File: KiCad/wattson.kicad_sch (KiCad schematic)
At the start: 24 parts, among them SW1 Keypad 1, SW10 Plug, SW11 On/Off, SW2 Keypad 2, SW3 Keypad 3, SW4 Keypad 4, SW5 Keypad 5, SW6 Keypad 0, SW7 Keypad 6, SW8 Keypad 7, SW9 Trigger, U1 CR2013-MI2120, U2 MCP23017_SO

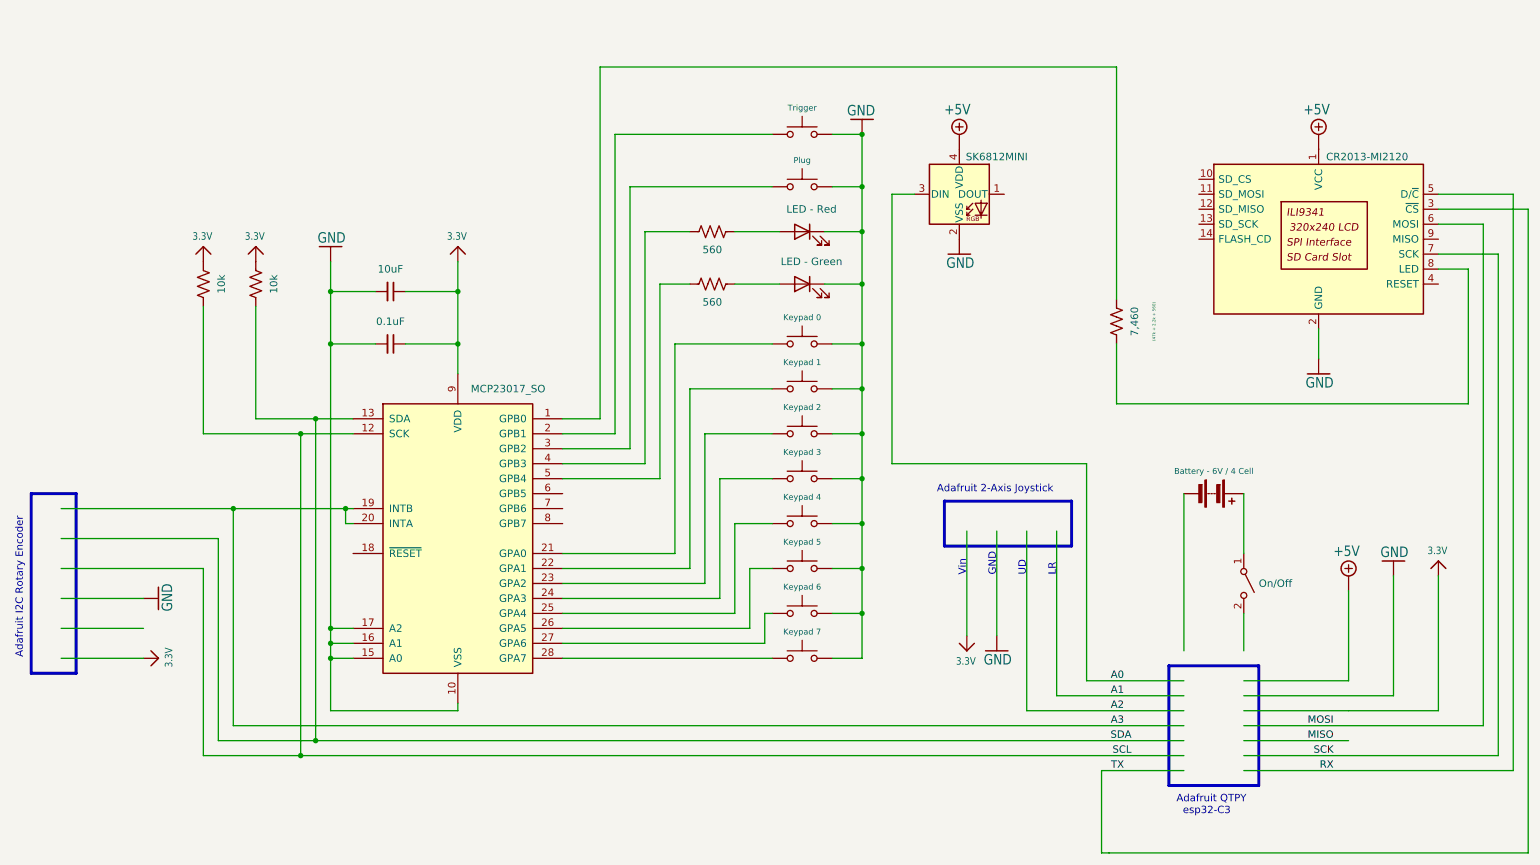
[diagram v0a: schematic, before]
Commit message: add vibration motors
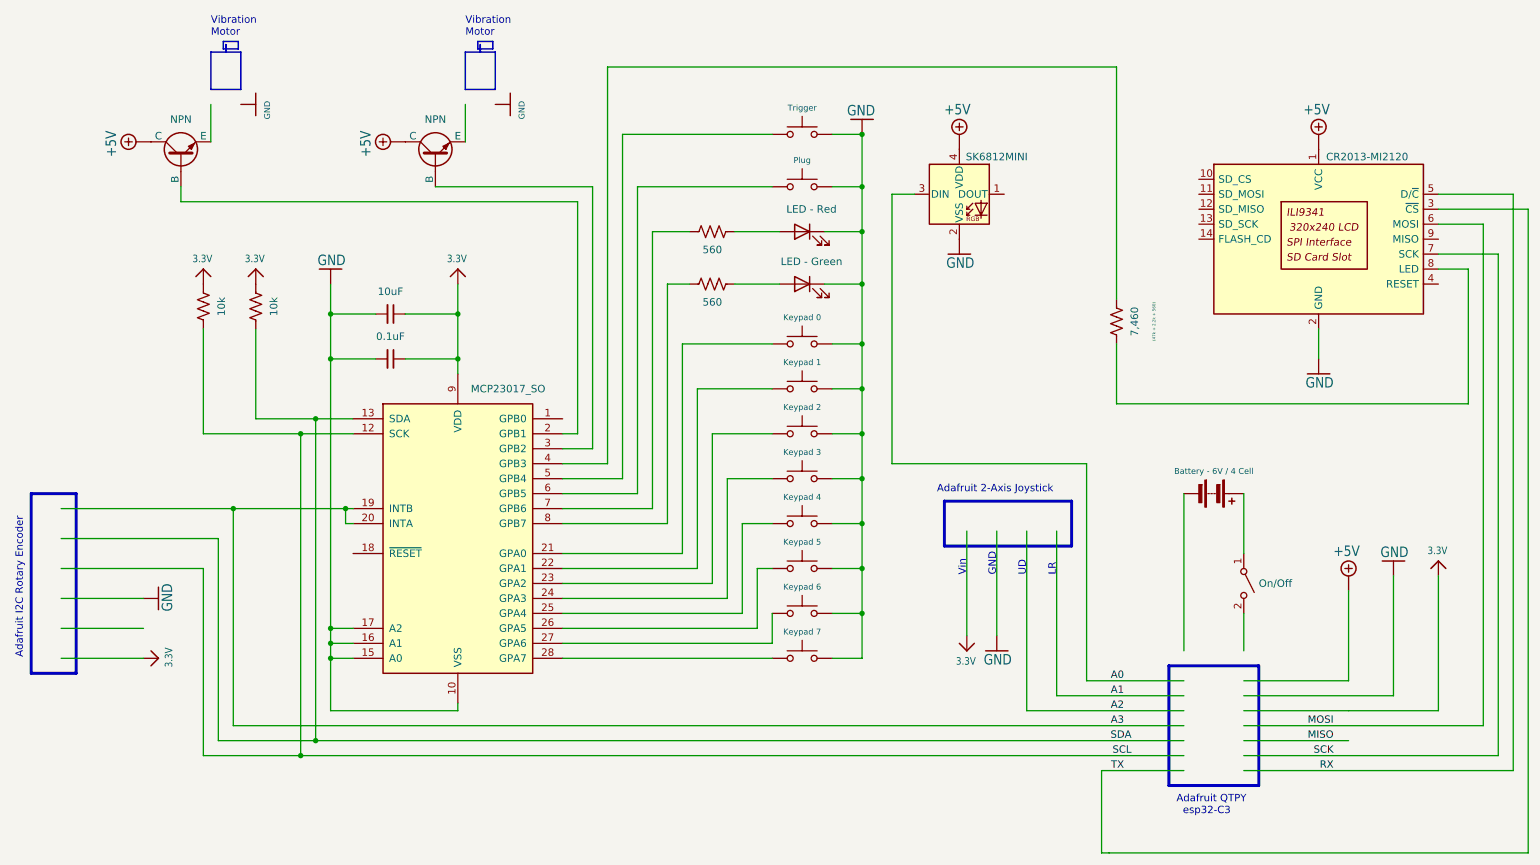
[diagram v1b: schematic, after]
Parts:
- added Q1, Q2: NPN, symbol Simulation_SPICE:NPN
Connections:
- net +5V: now also Q1.1 (C), Q2.1 (C)
- net at U2.1 (GPB0): no longer R6.1
- net at U2.2 (GPB1): now also Q1.2 (B); no longer SW9.1
- net at U2.3 (GPB2): now also Q2.2 (B); no longer SW10.1
- net at U2.4 (GPB3): now also R6.1; no longer R3.2
- net at U2.5 (GPB4): now also SW9.1; no longer R4.2
- net at U2.6 (GPB5): now also SW10.1
- net at U2.7 (GPB6): now also R3.2
- net at U2.8 (GPB7): now also R4.2
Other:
- note added: "Vibration Motor"
